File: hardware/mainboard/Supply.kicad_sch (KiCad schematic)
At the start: 18 parts, among them CN3 Header 7x2, U1 STM32WL33

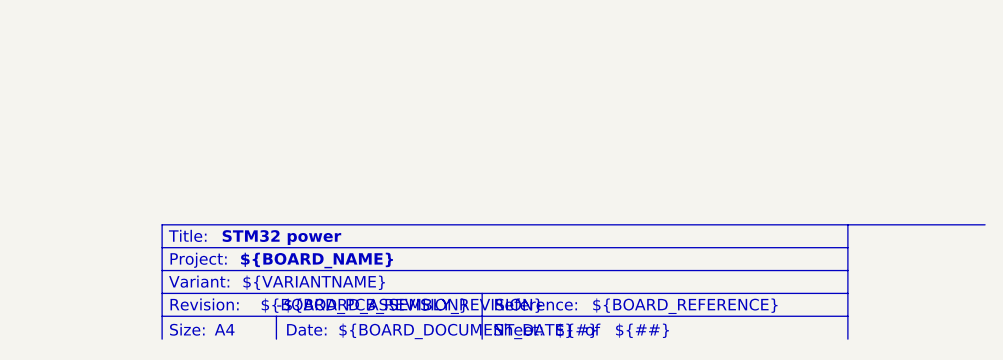
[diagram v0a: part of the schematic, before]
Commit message: latest
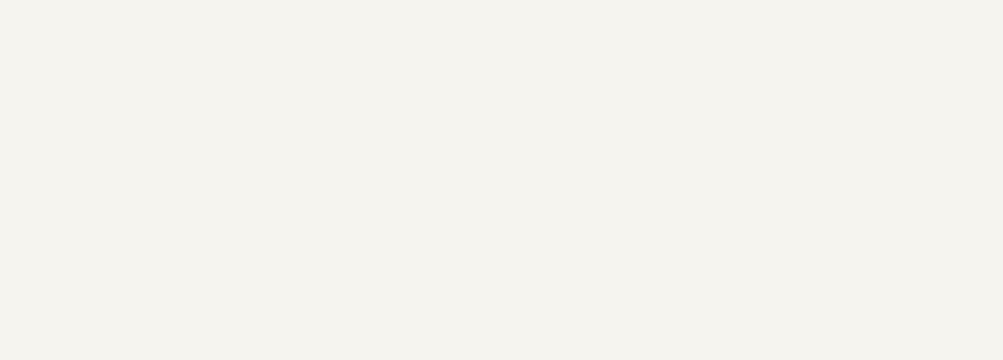
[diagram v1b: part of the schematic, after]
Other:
- note removed: "${##}"
- note removed: "${#}"
- note removed: "${BOARD_ASSEMBLY_REVISION}"
- note removed: "${BOARD_DOCUMENT_DATE}"
- note removed: "${BOARD_NAME}"
- note removed: "${BOARD_PCB_REVISION}"
- note removed: "${BOARD_REFERENCE}"
- note removed: "${TITLE}"
- note removed: "${VARIANTNAME}"
- note removed: "-"
- note removed: "A4"
- note removed: "Date:"
- note removed: "Project:"
- note removed: "Reference:"
- note removed: "Revision:"
- note removed: "Sheet:"
- note removed: "Size:"
- note removed: "Title:"
- note removed: "Variant:"
- note removed: "of"
